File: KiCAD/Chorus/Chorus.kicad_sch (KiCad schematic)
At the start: 86 parts, among them J1 IN, J2 OUT, J3 Conn_01x03, J4 Conn_01x03, Q1 BC337, Q2 BC337, SW1 SW_SPDT, U1 TL072, U2 TL072, U3 TL072, U4 PT2399, U5 L7805

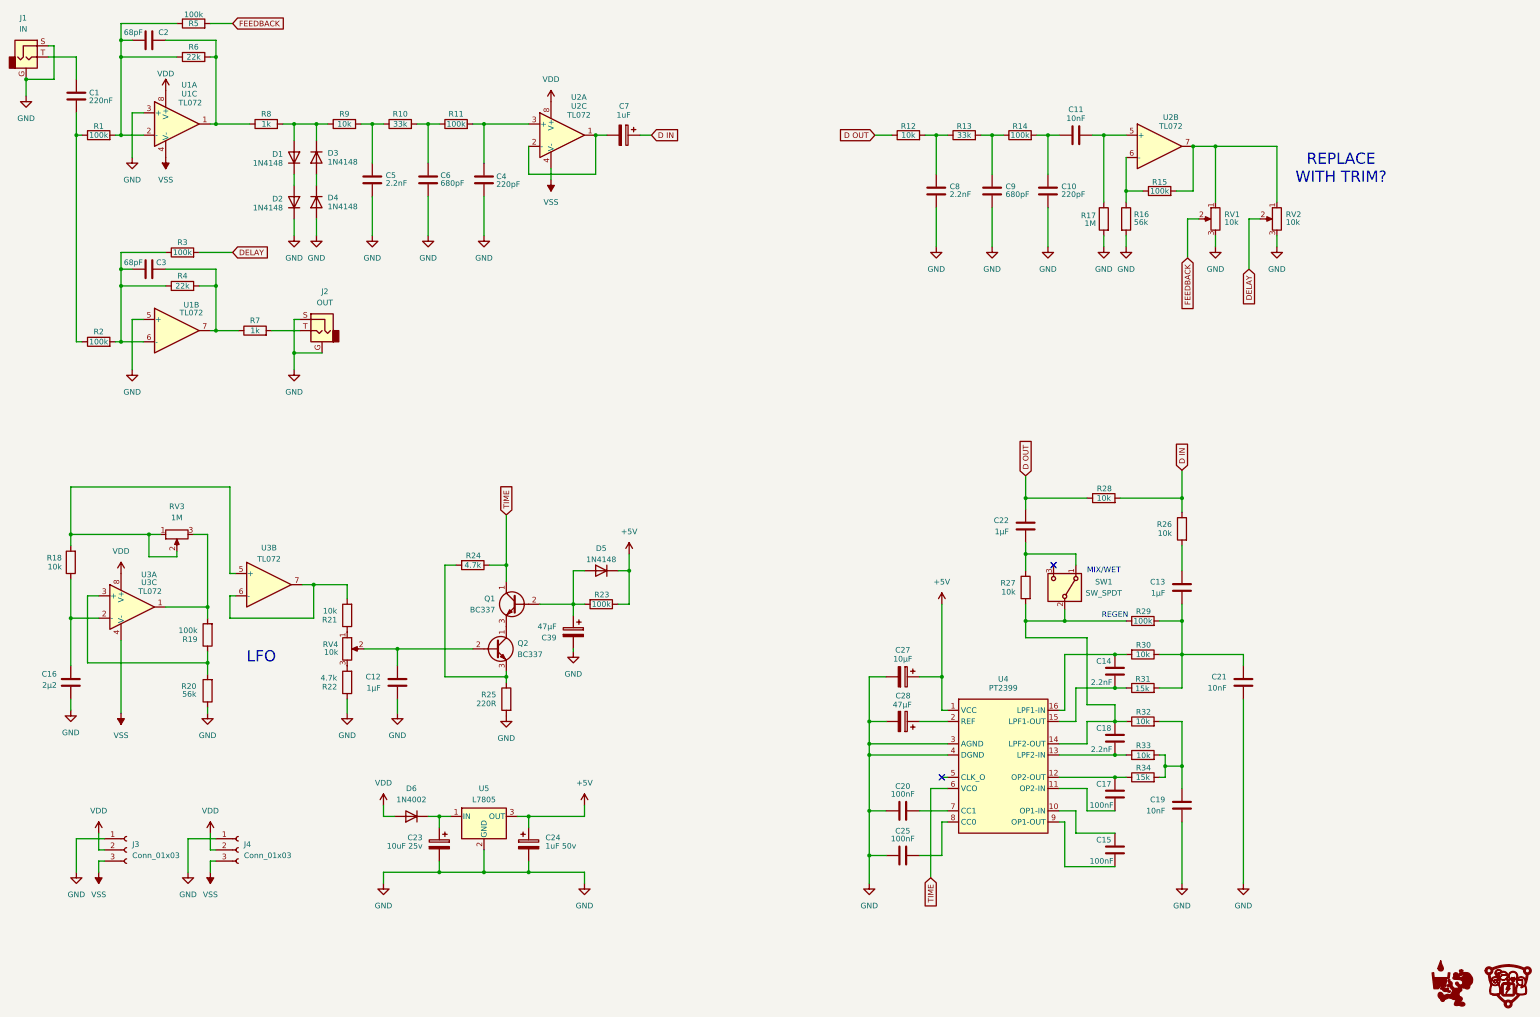
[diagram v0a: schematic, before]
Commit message: Chorus Trace v1
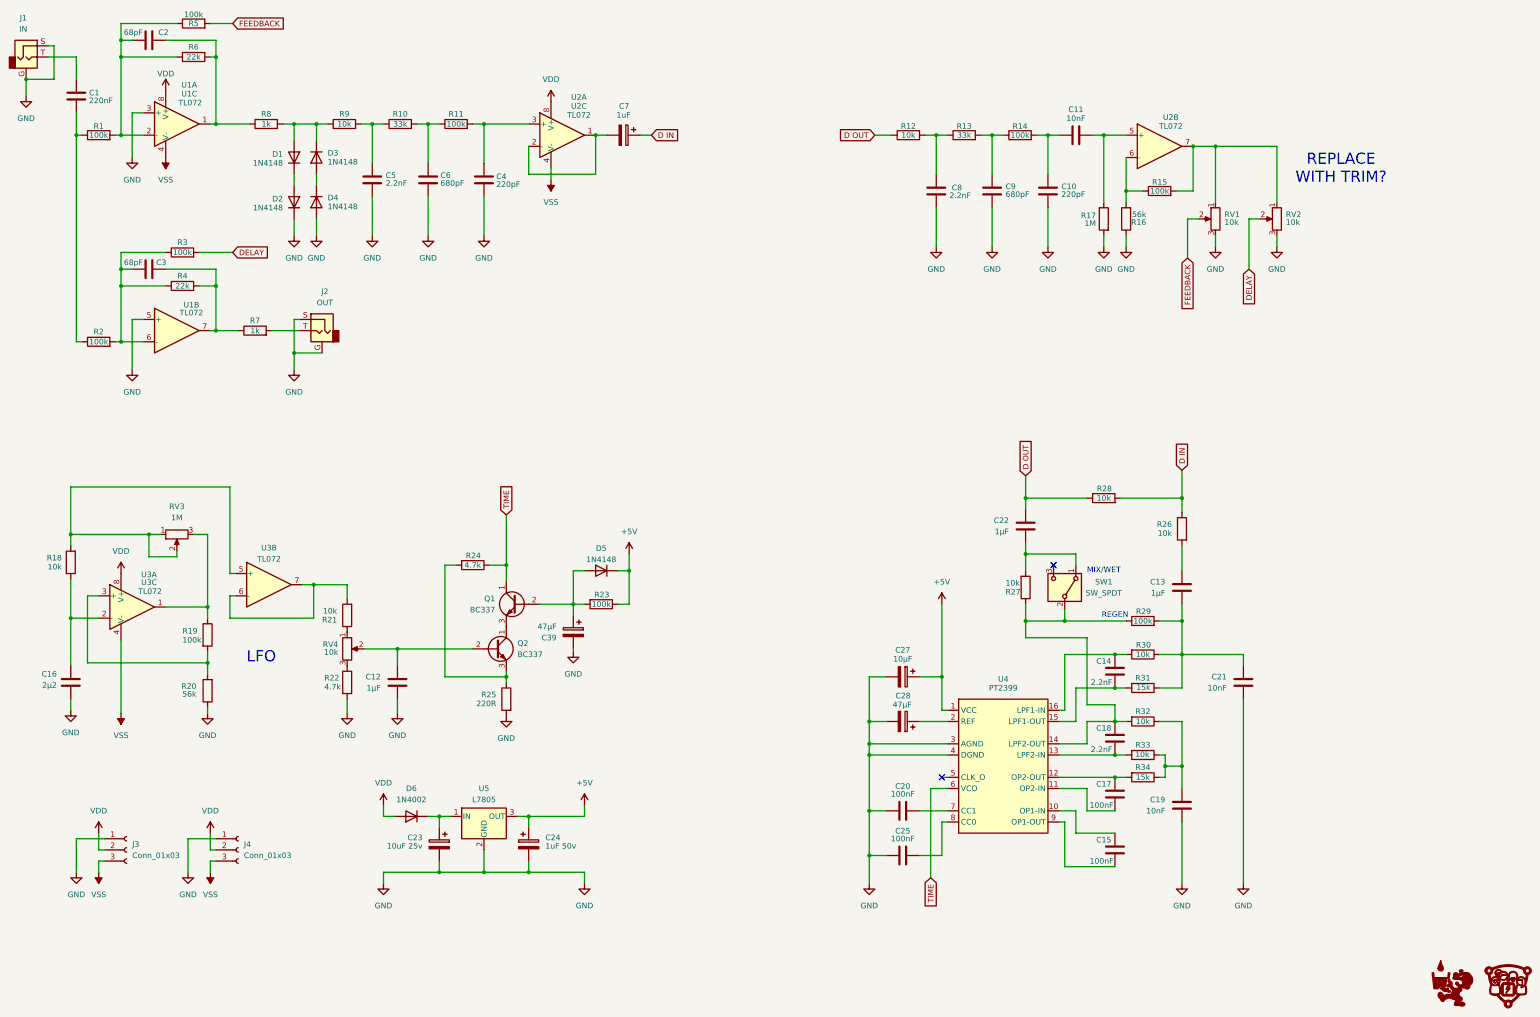
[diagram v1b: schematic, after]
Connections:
- net GND: now also C8.1, R16.1, R22.2; no longer C8.2, R16.2, R22.1
- net at R15.1, U2.6 (-): now also R16.2; no longer R16.1
- net at R12.2, R13.1: now also C8.2; no longer C8.1
- net at C22.2, SW1.1 (A): now also R27.2; no longer R27.1
- net at C18.1, R29.1, SW1.2 (B)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: now also R27.1, R32.2; no longer R27.2, R32.1
- net at R20.2, U3.3 (+): now also R19.2; no longer R19.1
- net at C13.2, C21.1, R29.2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: now also R31.1; no longer R31.2
- net at C17.1, U4.12 (OP2-OUT): now also R34.2; no longer R34.1
- net at C18.2, U4.13 (LPF2-IN): now also R33.2; no longer R33.1
- net at C14.2, U4.15 (LPF1-OUT): now also R31.2; no longer R31.1
- net at RV4.3: now also R22.1; no longer R22.2
- net at RV3.3, U3.1: now also R19.1; no longer R19.2
- new net: C19.1, R32.1, R33.1, R34.1
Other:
- moved on the sheet: R16, R19, R22, R31, R32, R33, R34
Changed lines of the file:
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@@
 	(symbol
 		(lib_id "HackSynth:R")
-		(at 312.42 86.36 0)
+		(at 312.42 86.36 180)
 		(unit 1)
 		(exclude_from_sim no)
@@
 		(dnp no)
 		(property "Reference" "R16"
-			(at 314.198 85.344 0)
+			(at 316.992 87.1221 0)
 			(effects
 				(font
@@
 		)
 		(property "Value" "56k"
-			(at 314.198 87.1221 0)
+			(at 316.992 85.344 0)
 			(effects
 				(font
@@
 		)
 		(property "Footprint" "HackSynth:R_Vertical_P2.54mm"
-			(at 310.642 86.36 90)
+			(at 314.198 86.36 90)
 			(effects
 				(font
@@
 		(lib_id "Device:C")
 		(at 269.24 80.01 0)
-		(mirror y)
+		(mirror x)
 		(unit 1)
 		(exclude_from_sim no)
@@
 		(dnp no)
 		(property "Reference" "C8"
-			(at 272.288 78.994 0)
+			(at 275.082 79.248 0)
 			(effects
 				(font
@@
 		)
 		(property "Value" "2.2nF"
-			(at 272.288 80.772 0)
+			(at 277.114 81.026 0)
 			(effects
 				(font
@@
 		)
 		(property "Footprint" "HackSynth:C_Ceramic_D4.5mm_P5.00mm"
-			(at 268.2748 83.82 0)
+			(at 270.2052 76.2 0)
 			(effects
 				(font
@@
 	(symbol
 		(lib_id "HackSynth:R")
-		(at 316.23 200.66 90)
+		(at 316.23 200.66 270)
 		(unit 1)
 		(exclude_from_sim no)
@@
 		(dnp no)
 		(property "Reference" "R32"
-			(at 316.357 198.501 90)
+			(at 316.23 198.374 90)
 			(effects
 				(font
@@
 		)
 		(property "Footprint" "HackSynth:R_Vertical_P2.54mm"
-			(at 316.23 202.438 90)
+			(at 316.23 198.882 90)
 			(effects
 				(font
@@
 	(symbol
 		(lib_id "HackSynth:R")
-		(at 316.23 213.36 90)
+		(at 316.23 213.36 270)
 		(unit 1)
 		(exclude_from_sim no)
@@
 		(dnp no)
 		(property "Reference" "R34"
-			(at 316.357 211.201 90)
+			(at 316.23 211.074 90)
 			(effects
 				(font
@@
 		)
 		(property "Footprint" "HackSynth:R_Vertical_P2.54mm"
-			(at 316.23 215.138 90)
+			(at 316.23 211.582 90)
 			(effects
 				(font
@@
 	(symbol
 		(lib_id "HackSynth:R")
-		(at 316.23 208.28 90)
+		(at 316.23 208.28 270)
 		(unit 1)
 		(exclude_from_sim no)
@@
 		(dnp no)
 		(property "Reference" "R33"
-			(at 316.357 206.121 90)
+			(at 316.23 205.994 90)
 			(effects
 				(font
@@
 		)
 		(property "Value" "10k"
-			(at 316.357 208.407 90)
+			(at 316.103 208.153 90)
 			(effects
 				(font
@@
 		)
 		(property "Footprint" "HackSynth:R_Vertical_P2.54mm"
-			(at 316.23 210.058 90)
+			(at 316.23 206.502 90)
 			(effects
 				(font
@@
 	(symbol
 		(lib_id "HackSynth:R")
-		(at 316.23 193.04 90)
+		(at 316.23 193.04 270)
 		(unit 1)
 		(exclude_from_sim no)
@@
 		(dnp no)
 		(property "Reference" "R31"
-			(at 316.23 191.008 90)
+			(at 316.23 190.754 90)
 			(effects
 				(font
@@
 		)
 		(property "Value" "15k"
-			(at 316.103 193.167 90)
+			(at 316.357 192.913 90)
 			(effects
 				(font
@@
 		)
 		(property "Footprint" "HackSynth:R_Vertical_P2.54mm"
-			(at 316.23 194.818 90)
+			(at 316.23 191.262 90)
 			(effects
 				(font
@@
 		(lib_id "HackSynth:R")
 		(at 289.56 170.18 0)
-		(mirror y)
+		(mirror x)
 		(unit 1)
 		(exclude_from_sim no)
@@
 		(dnp no)
 		(property "Reference" "R27"
-			(at 287.274 169.1639 0)
+			(at 284.988 171.1961 0)
 			(effects
 				(font
@@
 		)
 		(property "Value" "10k"
-			(at 287.274 171.196 0)
+			(at 284.988 169.164 0)
 			(effects
 				(font
@@
 		)
 		(property "Footprint" "HackSynth:R_Vertical_P2.54mm"
-			(at 291.338 170.18 90)
+			(at 287.782 170.18 90)
 			(effects
 				(font
@@
 	(symbol
 		(lib_id "HackSynth:R")
-		(at 103.505 180.975 180)
+		(at 103.505 180.975 0)
 		(unit 1)
 		(exclude_from_sim no)
@@
 		(dnp no)
 		(property "Reference" "R19"
-			(at 101.219 181.991 0)
+			(at 97.79 180.086 0)
 			(effects
 				(font
@@
 		)
 		(property "Value" "100k"
-			(at 101.219 179.9589 0)
+			(at 97.79 182.1181 0)
 			(effects
 				(font
@@
 		)
 		(property "Footprint" "HackSynth:R_Vertical_P2.54mm"
-			(at 105.283 180.975 90)
+			(at 101.727 180.975 90)
 			(effects
 				(font
@@
 	(symbol
 		(lib_id "HackSynth:R")
-		(at 135.255 191.77 180)
+		(at 135.255 191.77 0)
 		(unit 1)
 		(exclude_from_sim no)
@@
 		(dnp no)
 		(property "Reference" "R22"
-			(at 132.969 192.786 0)
+			(at 130.048 190.754 0)
 			(effects
 				(font
@@
 		)
 		(property "Value" "4.7k"
-			(at 132.969 190.7539 0)
+			(at 130.048 192.7861 0)
 			(effects
 				(font
@@
 		)
 		(property "Footprint" "HackSynth:R_Vertical_P2.54mm"
-			(at 137.033 191.77 90)
+			(at 133.477 191.77 90)
 			(effects
 				(font
